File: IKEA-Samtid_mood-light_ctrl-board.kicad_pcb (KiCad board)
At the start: 2 copper layers, 41.3 x 15.5 mm, 15 parts, among them IC1 ATMEGA168PA-M, P1 FTDI, P3.2 B-to-B-1B, P4.2 B-to-B-2B, SW1 ENTER, SW2 MODE, X1 CSTCE16M0V53-R0

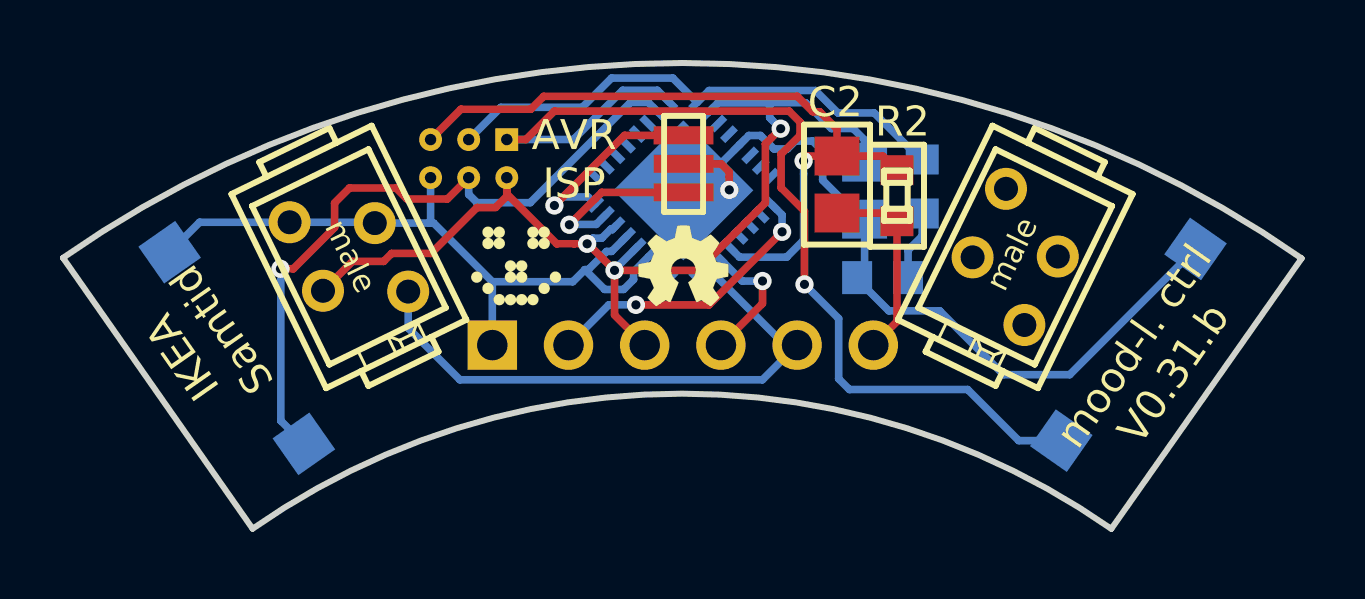
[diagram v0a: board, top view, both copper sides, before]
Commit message: Being creative...
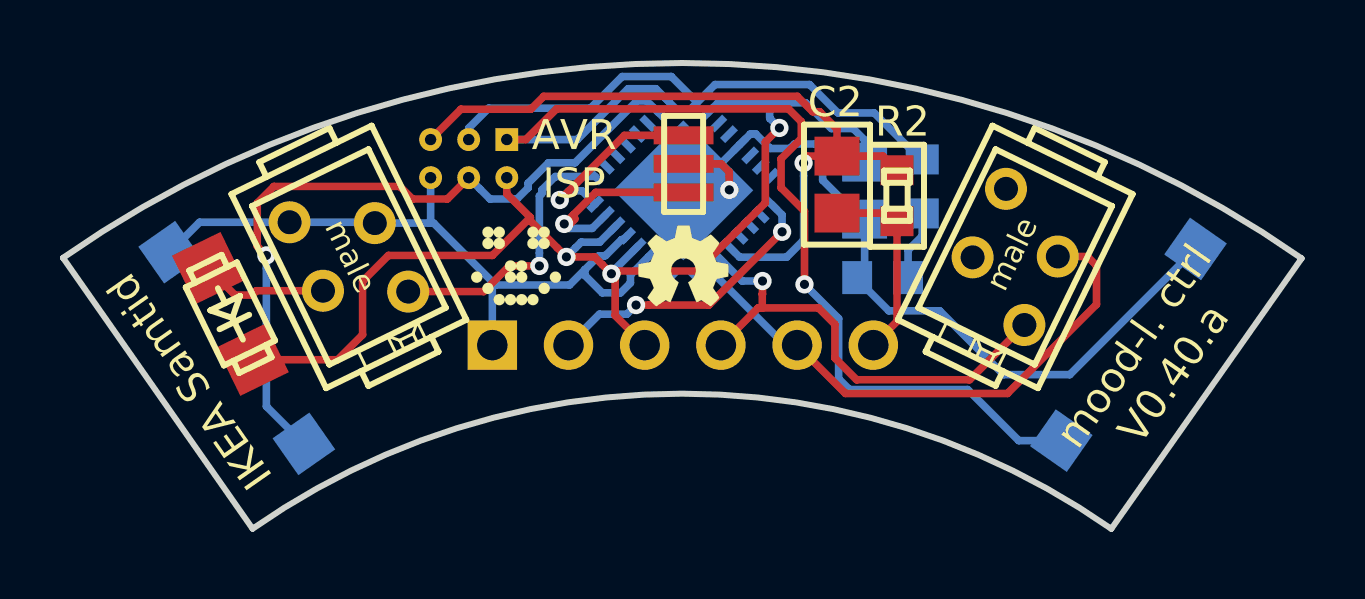
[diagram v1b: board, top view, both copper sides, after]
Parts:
- added DS1: DIODESCH, my_parts:MADW__diode_sub-SMA, F.Cu at (135.1, 95.6)
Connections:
- C1 pad 1: /VCC.B -> /VCC.B2
- IC1 pad 18: /VCC.B -> /VCC.B2
- IC1 pad 30: /RXI -> /RXI.B
- IC1 pad 31: /TXO -> /TXO.B
- IC1 pad 4: /VCC.B -> /VCC.B2
- IC1 pad 6: /VCC.B -> /VCC.B2
- IC1 pad 9: (no net) -> /LEDS.B
- JP1 pad 2: /VCC.B -> /VCC.B2
- P1 pad 3: /VCC.B -> /VCC.B2
- P1 pad 4: /RXI -> /RXI.B
- P1 pad 5: /TXO -> /TXO.B
- P3.2 pad 1: /TXO -> /LEDS.B
- P4.2 pad 1: (no net) -> /RXI.B
- P4.2 pad 3: (no net) -> /TXO.B
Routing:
- net /VCC.B2: track 0.00 -> 40.1 mm, vias 0 -> 3
- net /VCC.B: track 34.8 -> 4.26 mm, vias 3 -> 0
- net /TXO: track 19.4 -> 0.00 mm
- net /TXO.B: track 0.00 -> 18.6 mm
- net /RXI.B: track 0.00 -> 15.8 mm, vias 0 -> 1
- net /LEDS.B: track 0.00 -> 9.26 mm, vias 0 -> 1
- net /RXI: track 4.51 -> 0.00 mm, vias 1 -> 0
- net /MOSI: track 23.1 -> 24.7 mm
- net /XTAL1: track 5.93 -> 6.52 mm
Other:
- board text added: "mood-l. ctrl V0.40.a"
- board text removed: "mood-l. ctrl V0.31.b"
